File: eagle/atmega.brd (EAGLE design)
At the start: 82.4 x 66 mm, 65 parts, among them IC1 TO 5V, IC2 LM339D, Q2 16MHz, U1 ATMEGA328P-AU

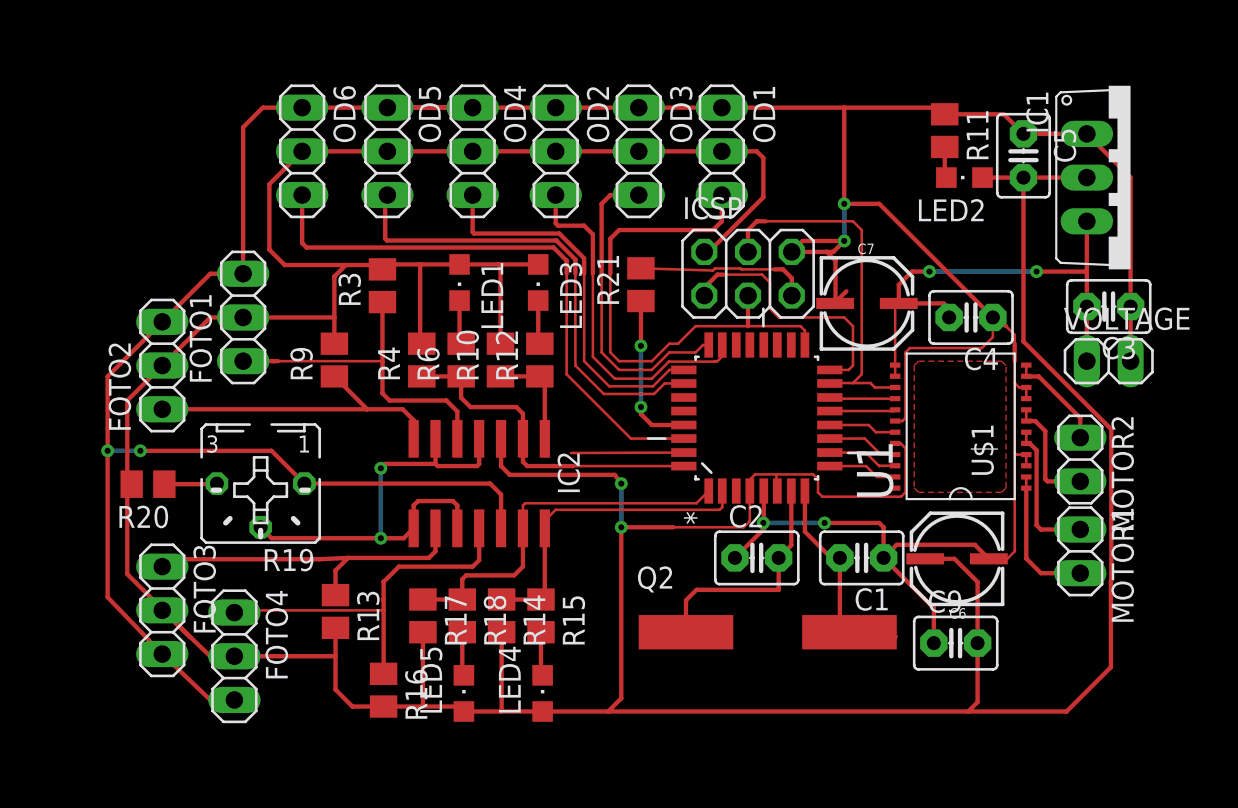
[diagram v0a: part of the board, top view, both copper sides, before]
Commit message: zapomiałem co się działo
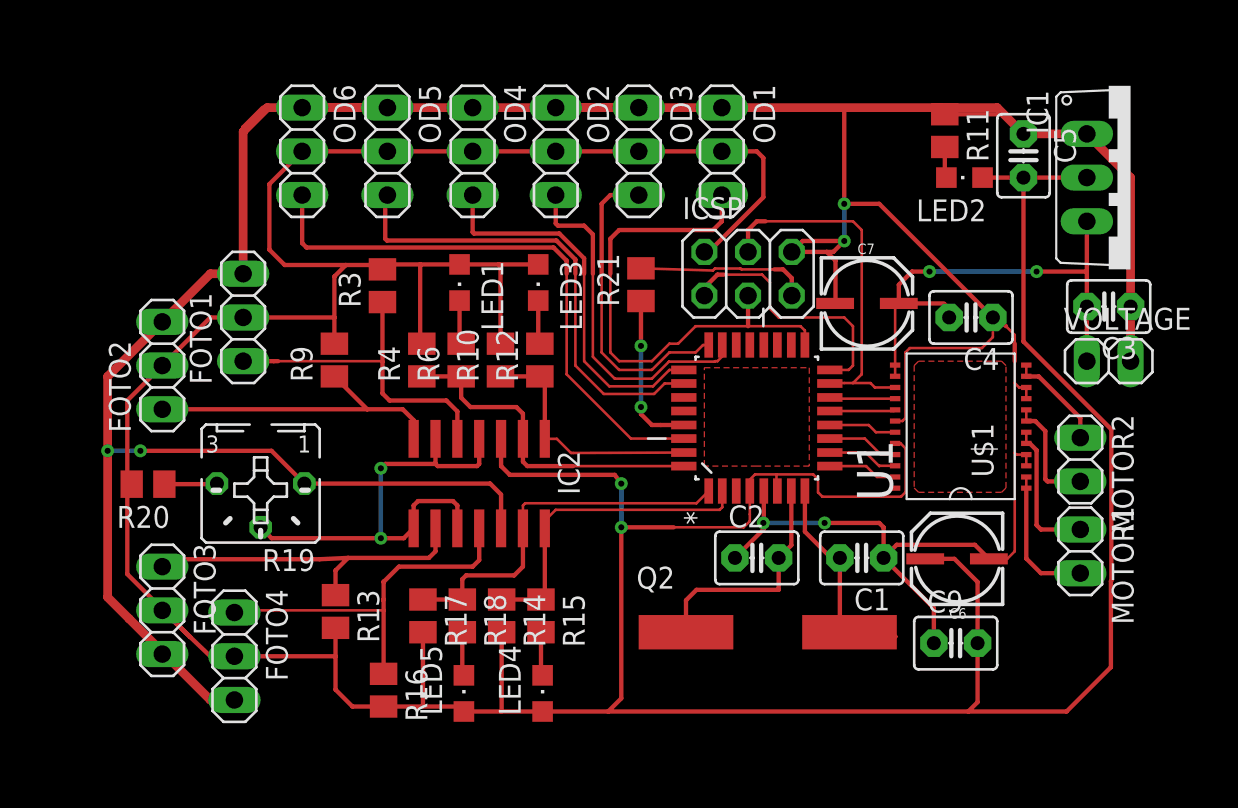
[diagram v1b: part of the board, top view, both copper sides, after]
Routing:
- net GND: track 223.2 -> 254.2 mm
- net KO2: track 12.6 -> 14.5 mm
- net PWMB: track 20.7 -> 21.3 mm
- added copper zone on layer 1, net N$5
